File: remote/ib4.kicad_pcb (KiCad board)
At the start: 4 copper layers, 96 x 77 mm, 15 parts, among them J1 Conn_01x02_Female, J2 Screw_Terminal_01x02, J3 Conn_01x07_Female, J6 Screw_Terminal_01x03, J7 Screw_Terminal_01x03, J8 Screw_Terminal_01x03, U2 tpl5110, U3 lora_breakout

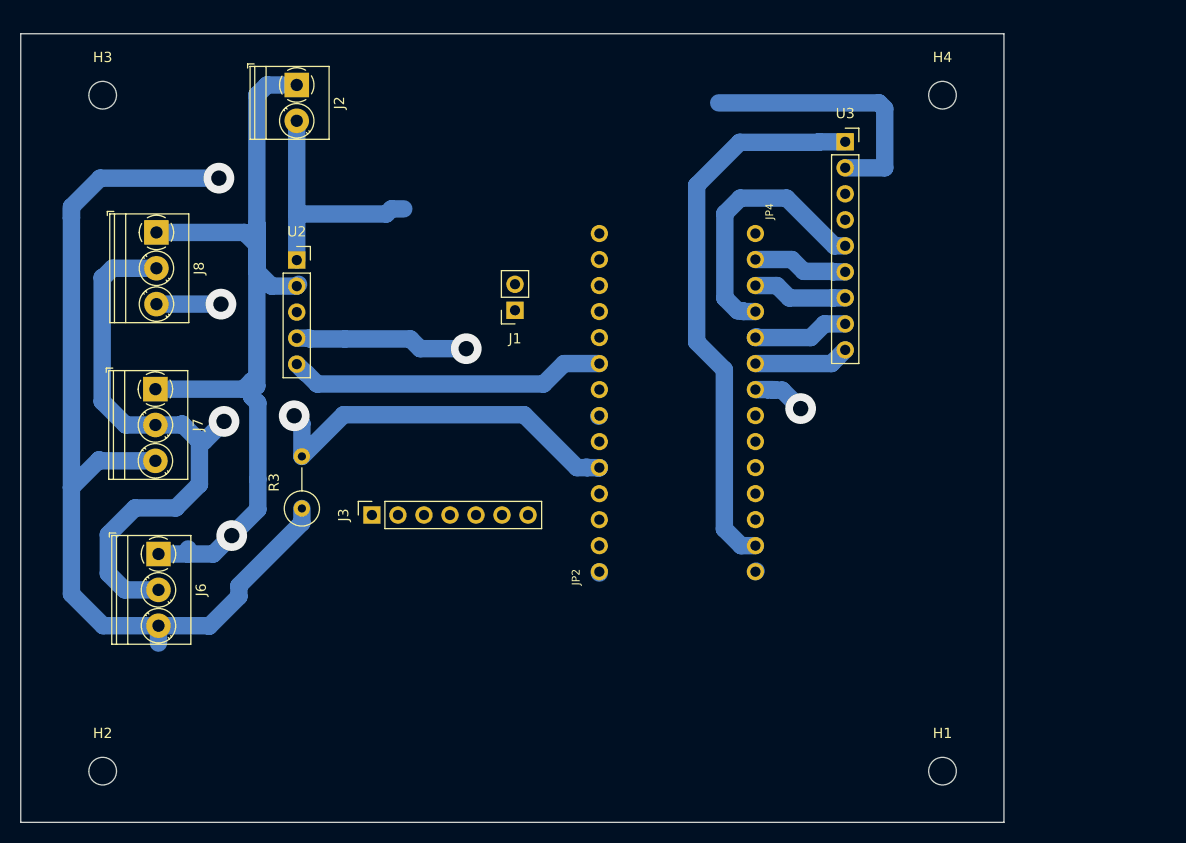
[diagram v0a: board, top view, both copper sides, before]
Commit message: update
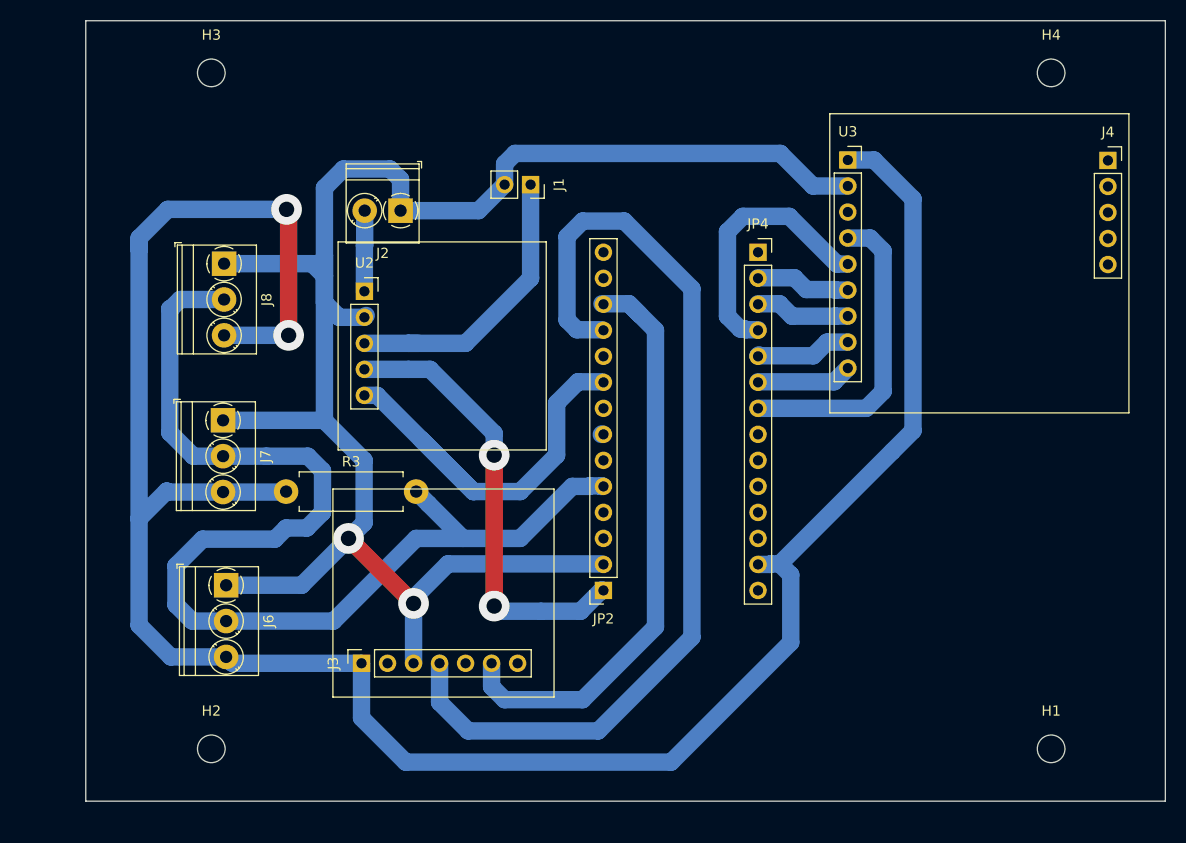
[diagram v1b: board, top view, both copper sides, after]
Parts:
- added J4: Conn_01x05_Female, Connector_PinSocket_2.54mm:PinSocket_1x05_P2.54mm_Vertical, F.Cu at (106.2, 12.4)
- JP2, JP4: footprint ib4:1X14_ROUND70 -> Connector_PinSocket_2.54mm:PinSocket_1x14_P2.54mm_Vertical
- R3: footprint Resistor_THT:R_Axial_DIN0309_L9.0mm_D3.2mm_P5.08mm_Vertical -> Resistor_THT:R_Axial_DIN0411_L9.9mm_D3.6mm_P12.70mm_Horizontal
- moved JP2 18.3 mm to (56.9, 54.4), turned to 180 degrees
- moved J2 15.9 mm to (37.1, 17.3), turned to 180 degrees
- moved JP4 14.7 mm to (72.0, 21.3), turned to 0 degrees
- moved J3 14.5 mm to (33.3, 61.5)
- moved J1 12.4 mm to (49.8, 14.7), turned to 270 degrees
- moved H2 10.8 mm to (18.6, 69.8)
- moved H3 10.8 mm to (18.6, 3.82)
- moved H1 10.8 mm to (100.6, 69.8)
- moved H4 10.8 mm to (100.6, 3.82)
- moved U2 7.27 mm to (33.6, 25.1)
- moved J6 7.27 mm to (20.1, 53.8)
- moved J8 7.27 mm to (19.9, 22.4)
- moved J7 7.27 mm to (19.8, 37.7)
- moved R3 2.26 mm to (25.9, 44.7), turned to 0 degrees
- moved U3 1.80 mm to (80.8, 12.3)
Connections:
- JP4 pad 7: (no net) -> G0
- U3 pad 4: (no net) -> G0
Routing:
- net SCL: track 0.00 -> 94.9 mm
- net +3V3: track 156.3 -> 224.8 mm
- net GND: track 113.7 -> 175.4 mm, vias 1 -> 2
- net SDA: track 0.00 -> 58.5 mm
- net G0: track 0.00 -> 30.6 mm
- net Net-(J1-Pad1): track 0.00 -> 29.0 mm
- net TIMED_POWER: track 17.1 -> 43.8 mm, vias 1 -> 2
- net D12: track 94.0 -> 112.9 mm, vias 2 -> 0
- net LI-ION: track 24.3 -> 7.89 mm
- net DONE: track 31.2 -> 41.7 mm
- net (no net): track 6.09 -> 0.09 mm, vias 1 -> 0
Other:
- board size 96 x 77 mm -> 105.4 x 76.2 mm
